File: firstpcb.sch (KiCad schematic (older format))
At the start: 10 parts

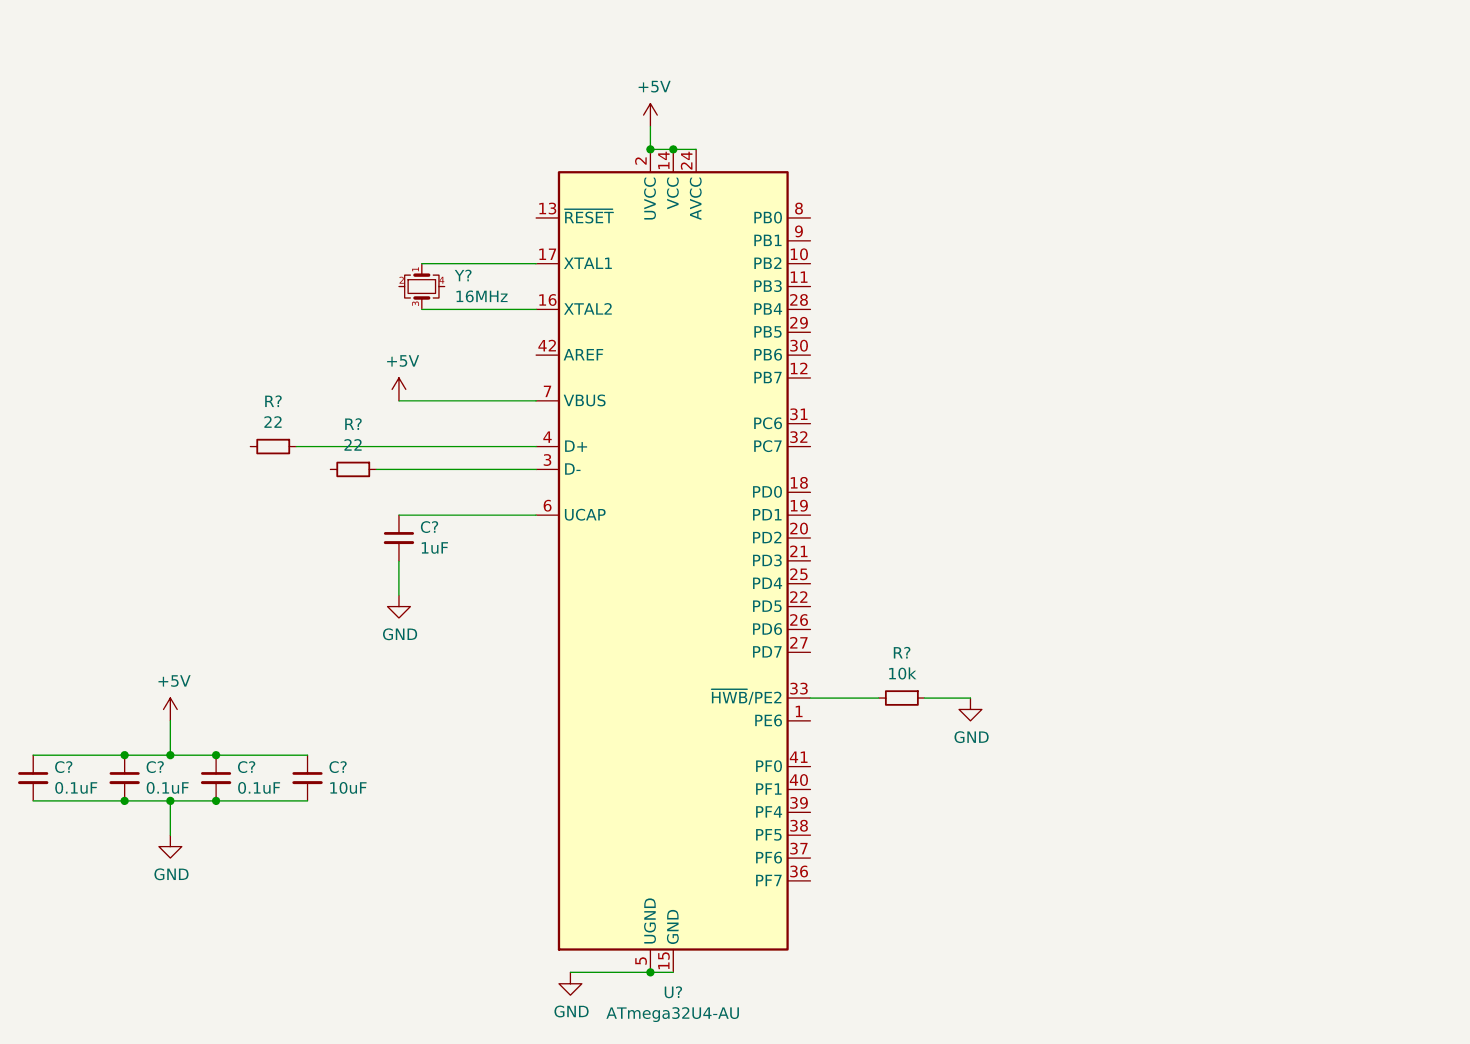
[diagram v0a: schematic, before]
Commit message: shematic
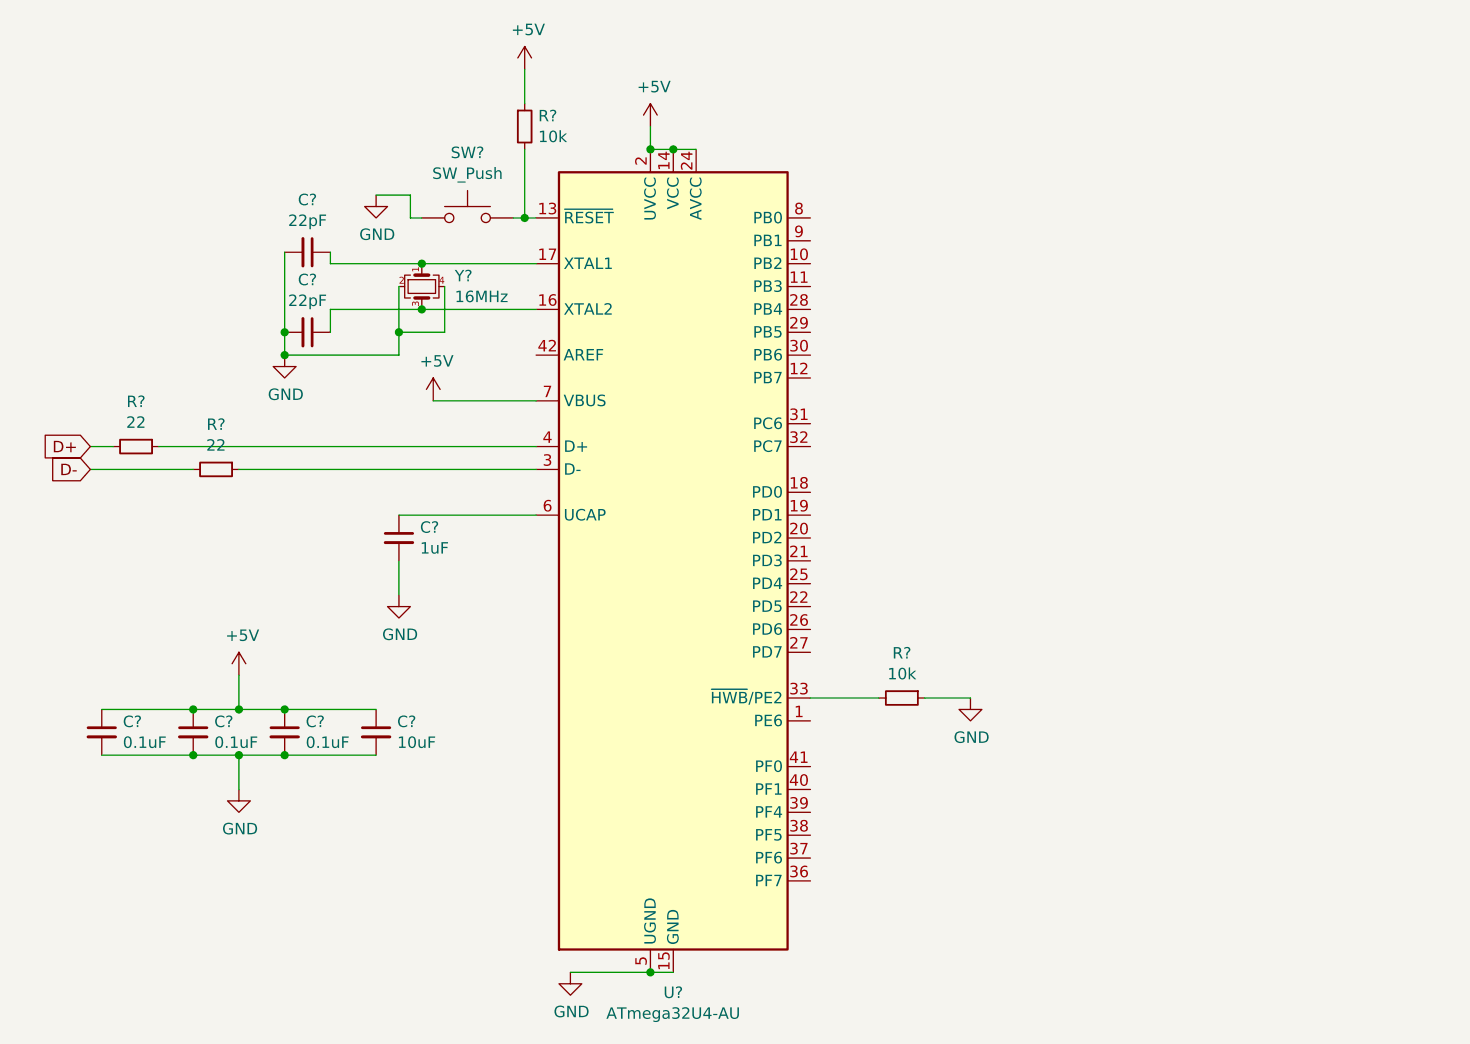
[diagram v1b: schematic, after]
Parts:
- added C? (x2): 22pF, symbol Device:C_Small
- added R?: 10k, symbol Device:R_Small
- added SW?: SW_Push, symbol Switch:SW_Push
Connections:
- net +5V: now also R?.1
- net GND: now also Y?.2, Y?.4, C?.2, C?.2, SW?.1
- net at U?.13 (~RESET): now also R?.2, SW?.2
- net at U?.16 (XTAL2), Y?.3: now also C?.1
- net at U?.17 (XTAL1), Y?.1: now also C?.1
- net D-: now reaches R?.2
- net D+: now reaches R?.2
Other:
- moved on the sheet: C?, R?

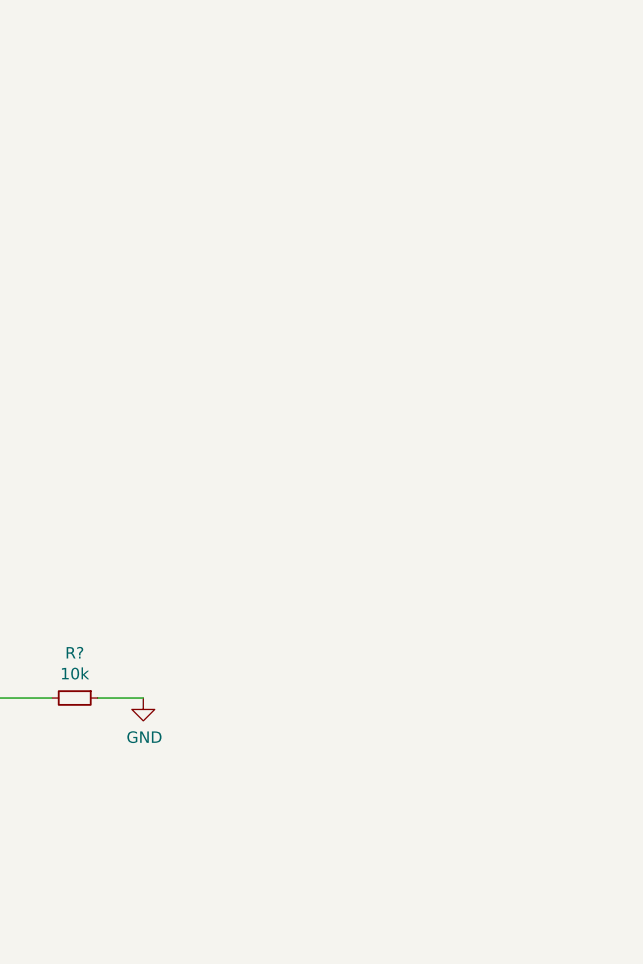
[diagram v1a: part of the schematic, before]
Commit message: schematic
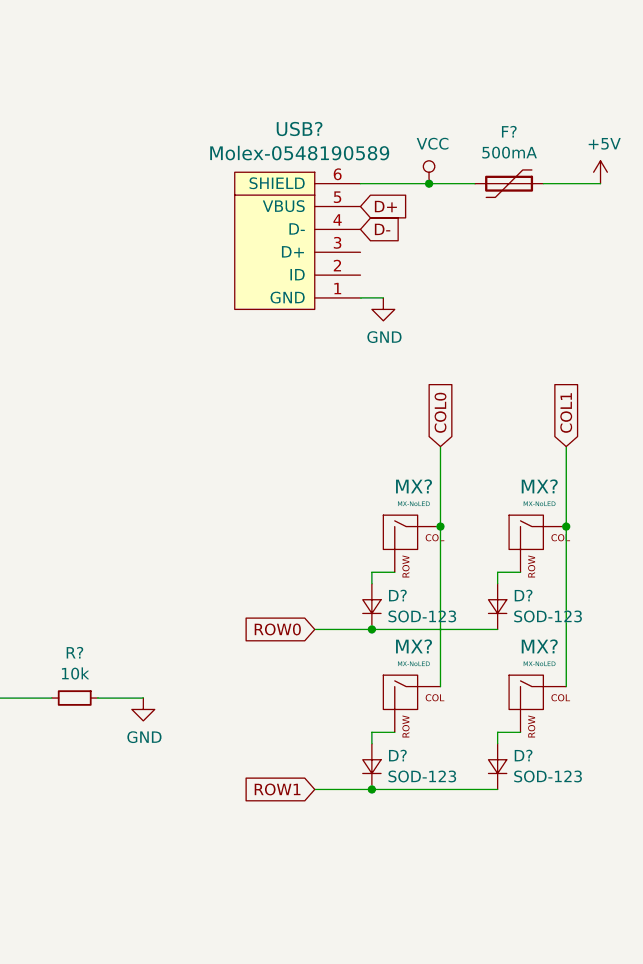
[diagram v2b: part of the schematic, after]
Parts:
- added D? (x4): SOD-123, symbol Device:D_Small
- added F?: 500mA, symbol Device:Polyfuse
- added MX? (x4): MX-NoLED, symbol MX_Alps_Hybrid:MX-NoLED
- added USB?: Molex-0548190589, symbol random-keyboard-parts:Molex-0548190589
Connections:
- net +5V: now also F?.1
- net D+: now also USB?.5 (VBUS)
- net D-: now also USB?.4 (D-)
- net GND: now also USB?.1 (GND)
- new net: D?.2 (A), MX?.2 (ROW) (x4)
- new net COL0: MX?.1 (COL), MX?.1 (COL)
- new net COL1: MX?.1 (COL), MX?.1 (COL)
- new net ROW0: D?.1 (K), D?.1 (K)
- new net ROW1: D?.1 (K), D?.1 (K)
- new net VCC: F?.2, USB?.6 (SHIELD)
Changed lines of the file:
@@
 Wire Wire Line
 	2700 3000 2250 3000
+$Comp
+L random-keyboard-parts:Molex-0548190589 USB?
+U 1 1 636BF531
+P 6750 2050
+F 0 "USB?" V 7287 2017 60  0000 C CNN
+F 1 "Molex-0548190589" V 7181 2017 60  0000 C CNN
+F 2 "" H 6750 2050 60  0001 C CNN
+F 3 "" H 6750 2050 60  0001 C CNN
+	1    6750 2050
+	0    -1   -1   0
+$EndComp
+$Comp
+L power:VCC #PWR?
+U 1 1 636C0166
+P 7350 1750
+F 0 "#PWR?" H 7350 1600 50  0001 C CNN
+F 1 "VCC" H 7367 1923 50  0000 C CNN
+F 2 "" H 7350 1750 50  0001 C CNN
+F 3 "" H 7350 1750 50  0001 C CNN
+	1    7350 1750
+	1    0    0    -1
+$EndComp
+$Comp
+L Device:Polyfuse F?
+U 1 1 636C3A9A
+P 7700 1750
+F 0 "F?" V 7475 1750 50  0000 C CNN
+F 1 "500mA" V 7566 1750 50  0000 C CNN
+F 2 "" H 7750 1550 50  0001 L CNN
+F 3 "~" H 7700 1750 50  0001 C CNN
+	1    7700 1750
+	0    1    1    0
+$EndComp
+$Comp
+L power:+5V #PWR?
+U 1 1 636C5D2B
+P 8100 1750
+F 0 "#PWR?" H 8100 1600 50  0001 C CNN
+F 1 "+5V" H 8115 1923 50  0000 C CNN
+F 2 "" H 8100 1750 50  0001 C CNN
+F 3 "" H 8100 1750 50  0001 C CNN
+	1    8100 1750
+	1    0    0    -1
+$EndComp
+Wire Wire Line
+	7050 1750 7350 1750
+Wire Wire Line
+	7850 1750 8100 1750
+Connection ~ 7350 1750
+Wire Wire Line
+	7350 1750 7550 1750
+$Comp
+L power:GND #PWR?
+U 1 1 636C745E
+P 7150 2250
+F 0 "#PWR?" H 7150 2000 50  0001 C CNN
+F 1 "GND" H 7155 2077 50  0000 C CNN
+F 2 "" H 7150 2250 50  0001 C CNN
+F 3 "" H 7150 2250 50  0001 C CNN
+	1    7150 2250
+	1    0    0    -1
+$EndComp
+Text GLabel 7050 1950 2    50   Input ~ 0
+D-
+Text GLabel 7050 1850 2    50   Input ~ 0
+D+
+Wire Wire Line
+	7050 2250 7150 2250
+$Comp
+L MX_Alps_Hybrid:MX-NoLED MX?
+U 1 1 636E001D
+P 7250 3300
+F 0 "MX?" H 7283 3523 60  0000 C CNN
+F 1 "MX-NoLED" H 7283 3449 20  0000 C CNN
+F 2 "" H 6625 3275 60  0001 C CNN
+F 3 "" H 6625 3275 60  0001 C CNN
+	1    7250 3300
+	1    0    0    -1
+$EndComp
+$Comp
+L Device:D_Small D?
+U 1 1 636EA45A
+P 7100 3600
+F 0 "D?" V 7146 3532 50  0000 R CNN
+F 1 "SOD-123" V 7055 3532 50  0000 R CNN
+F 2 "" V 7100 3600 50  0001 C CNN
+F 3 "~" V 7100 3600 50  0001 C CNN
+	1    7100 3600
+	0    -1   -1   0
+$EndComp
+Wire Wire Line
+	7200 3450 7100 3450
+Wire Wire Line
+	7100 3450 7100 3500
+$Comp
+L MX_Alps_Hybrid:MX-NoLED MX?
+U 1 1 636F0FB9
+P 7800 3300
+F 0 "MX?" H 7833 3523 60  0000 C CNN
+F 1 "MX-NoLED" H 7833 3449 20  0000 C CNN
+F 2 "" H 7175 3275 60  0001 C CNN
+F 3 "" H 7175 3275 60  0001 C CNN
+	1    7800 3300
+	1    0    0    -1
+$EndComp
+$Comp
+L Device:D_Small D?
+U 1 1 636F0FBF
+P 7650 3600
+F 0 "D?" V 7696 3532 50  0000 R CNN
+F 1 "SOD-123" V 7605 3532 50  0000 R CNN
+F 2 "" V 7650 3600 50  0001 C CNN
+F 3 "~" V 7650 3600 50  0001 C CNN
+	1    7650 3600
+	0    -1   -1   0
+$EndComp
+Wire Wire Line
+	7750 3450 7650 3450
+Wire Wire Line
+	7650 3450 7650 3500
+$Comp
+L MX_Alps_Hybrid:MX-NoLED MX?
+U 1 1 636F86FE
+P 7250 4000
+F 0 "MX?" H 7283 4223 60  0000 C CNN
+F 1 "MX-NoLED" H 7283 4149 20  0000 C CNN
+F 2 "" H 6625 3975 60  0001 C CNN
+F 3 "" H 6625 3975 60  0001 C CNN
+	1    7250 4000
+	1    0    0    -1
+$EndComp
+$Comp
+L Device:D_Small D?
+U 1 1 636F8704
+P 7100 4300
+F 0 "D?" V 7146 4232 50  0000 R CNN
+F 1 "SOD-123" V 7055 4232 50  0000 R CNN
+F 2 "" V 7100 4300 50  0001 C CNN
+F 3 "~" V 7100 4300 50  0001 C CNN
+	1    7100 4300
+	0    -1   -1   0
+$EndComp
+Wire Wire Line
+	7200 4150 7100 4150
+Wire Wire Line
+	7100 4150 7100 4200
+$Comp
+L MX_Alps_Hybrid:MX-NoLED MX?
+U 1 1 636F870C
+P 7800 4000
+F 0 "MX?" H 7833 4223 60  0000 C CNN
+F 1 "MX-NoLED" H 7833 4149 20  0000 C CNN
+F 2 "" H 7175 3975 60  0001 C CNN
+F 3 "" H 7175 3975 60  0001 C CNN
+	1    7800 4000
+	1    0    0    -1
+$EndComp
+$Comp
+L Device:D_Small D?
+U 1 1 636F8712
+P 7650 4300
+F 0 "D?" V 7696 4232 50  0000 R CNN
+F 1 "SOD-123" V 7605 4232 50  0000 R CNN
+F 2 "" V 7650 4300 50  0001 C CNN
+F 3 "~" V 7650 4300 50  0001 C CNN
+	1    7650 4300
+	0    -1   -1   0
+$EndComp
+Wire Wire Line
+	7750 4150 7650 4150
+Wire Wire Line
+	7650 4150 7650 4200
+Wire Wire Line
+	7950 2900 7950 3250
+Connection ~ 7950 3250
+Wire Wire Line
+	7950 3250 7950 3950
+Wire Wire Line
+	7400 2900 7400 3250
+Connection ~ 7400 3250
+Wire Wire Line
+	7400 3250 7400 3950
+Wire Wire Line
+	6850 3700 7100 3700
+Connection ~ 7100 3700
+Wire Wire Line
+	7100 3700 7650 3700
+Wire Wire Line
+	6850 4400 7100 4400
+Connection ~ 7100 4400
+Wire Wire Line
+	7100 4400 7650 4400
+Text GLabel 7400 2900 1    50   Input ~ 0
+COL0
+Text GLabel 7950 2900 1    50   Input ~ 0
+COL1
+Text GLabel 6850 3700 0    50   Input ~ 0
+ROW0
+Text GLabel 6850 4400 0    50   Input ~ 0
+ROW1
 $EndSCHEMATC
